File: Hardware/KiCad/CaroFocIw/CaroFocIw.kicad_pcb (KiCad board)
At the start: 4 copper layers, 85 x 42 mm, 100 parts, among them J1 Conn_01x04, J10 Conn_01x03, J11 Conn_01x03, J12 Conn_01x03, J13 Conn_01x04, J14 Conn_01x04, J15 Conn_01x04, J16 Conn_01x04, J17 Conn_01x04, J18 Conn_01x04, J19 Conn_01x02, J2 Conn_01x01, J20 Conn_01x02, J3 Conn_01x01, J4 Conn_01x04_MountingPin, J5 Conn_01x02, J6 Conn_01x02, J7 Conn_01x03, J8 Conn_01x03, J9 Conn_01x03, Q1 BSZ013NE2LS5I, Q2 BSZ013NE2LS5I, Q3 BSZ013NE2LS5I, Q4 BSZ013NE2LS5I, Q5 BSZ013NE2LS5I, Q6 BSZ013NE2LS5I, U1 Conn_01x01, U2 TCAN332, U3 STM32F405RGTx, U4 TLE7185-1E, U5 ACS711xEXLT-15AB, U6 AS5048A, U7 ACS711xEXLT-15AB, U8 ACS711xEXLT-15AB, U9 LMR16006YQ3

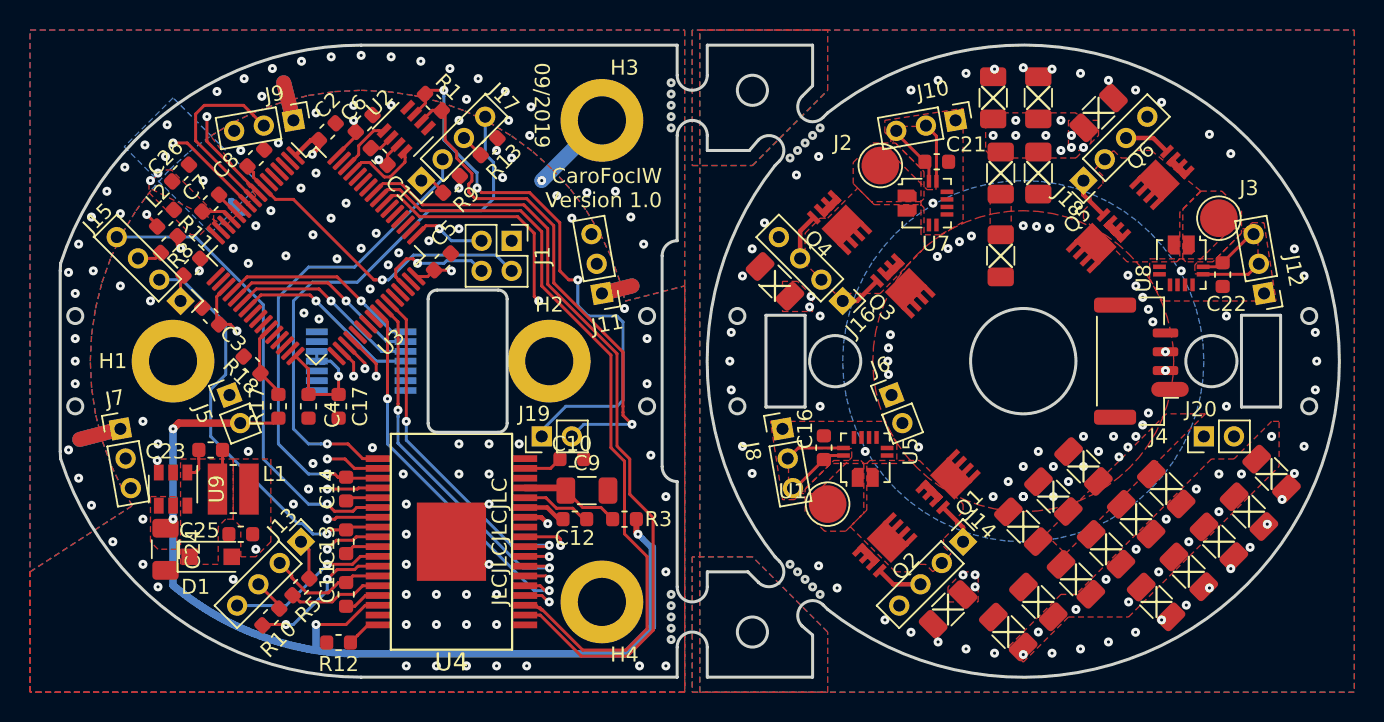
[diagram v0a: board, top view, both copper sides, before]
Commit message: Actual actual version 1.0, some minor changes. PCBs ordered.
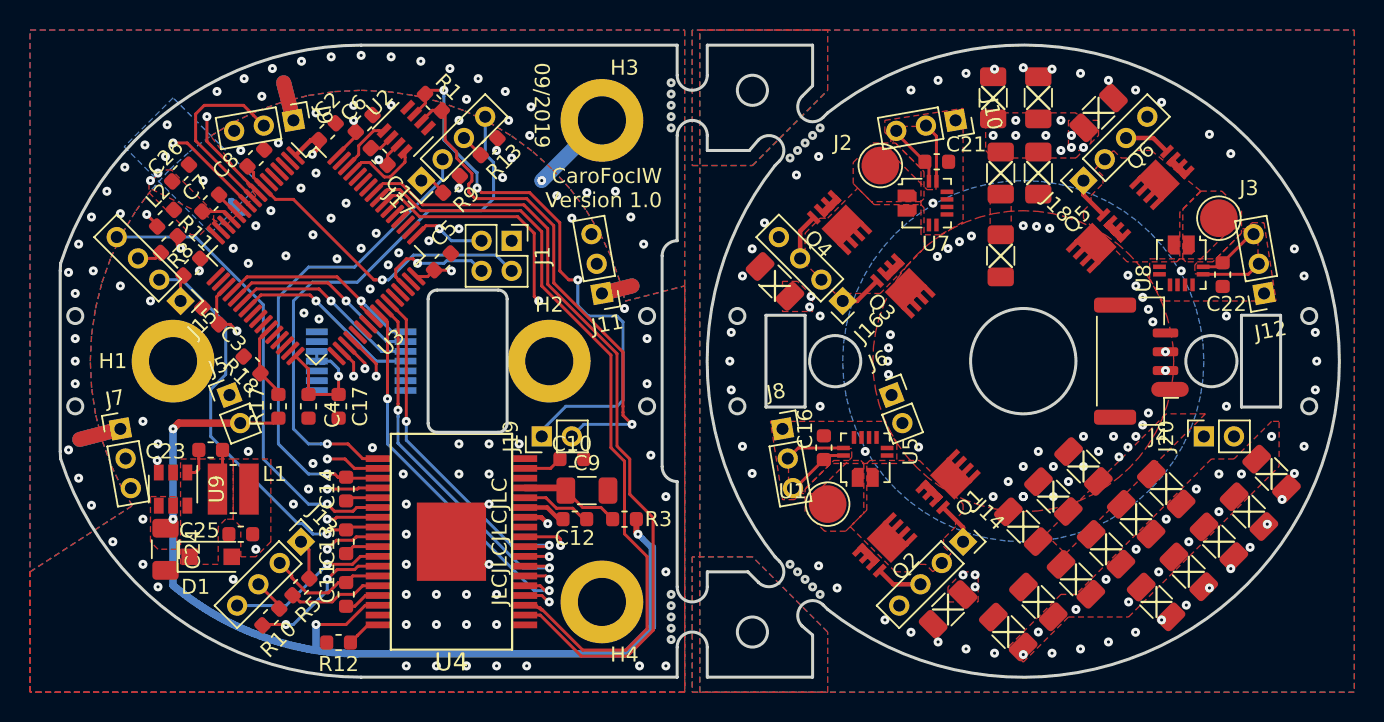
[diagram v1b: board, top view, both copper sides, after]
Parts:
- J10, J12, J8: footprint Connector_PinHeader_2.00mm:PinHeader_1x03_P2.00mm_Vertical -> Connector_PinSocket_2.00mm:PinSocket_1x03_P2.00mm_Vertical
- J14, J16, J18: footprint Connector_PinHeader_2.00mm:PinHeader_1x04_P2.00mm_Vertical -> Connector_PinSocket_2.00mm:PinSocket_1x04_P2.00mm_Vertical
- J20, J6: footprint Connector_PinHeader_2.00mm:PinHeader_1x02_P2.00mm_Vertical -> Connector_PinSocket_2.00mm:PinSocket_1x02_P2.00mm_Vertical
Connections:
- U3 pad 40: (no net) -> /Encoder/~EncoderCs
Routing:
- net /Encoder/~EncoderCs: track 13.5 -> 15.0 mm
